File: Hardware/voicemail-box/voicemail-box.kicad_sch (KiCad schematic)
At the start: 13 parts, among them J1 Power, J2 Digital/PWM, J3 Analog, J4 Digital/PWM, J5 Conn_02x06_Top_Bottom, U1 ESP32-WROOM-32

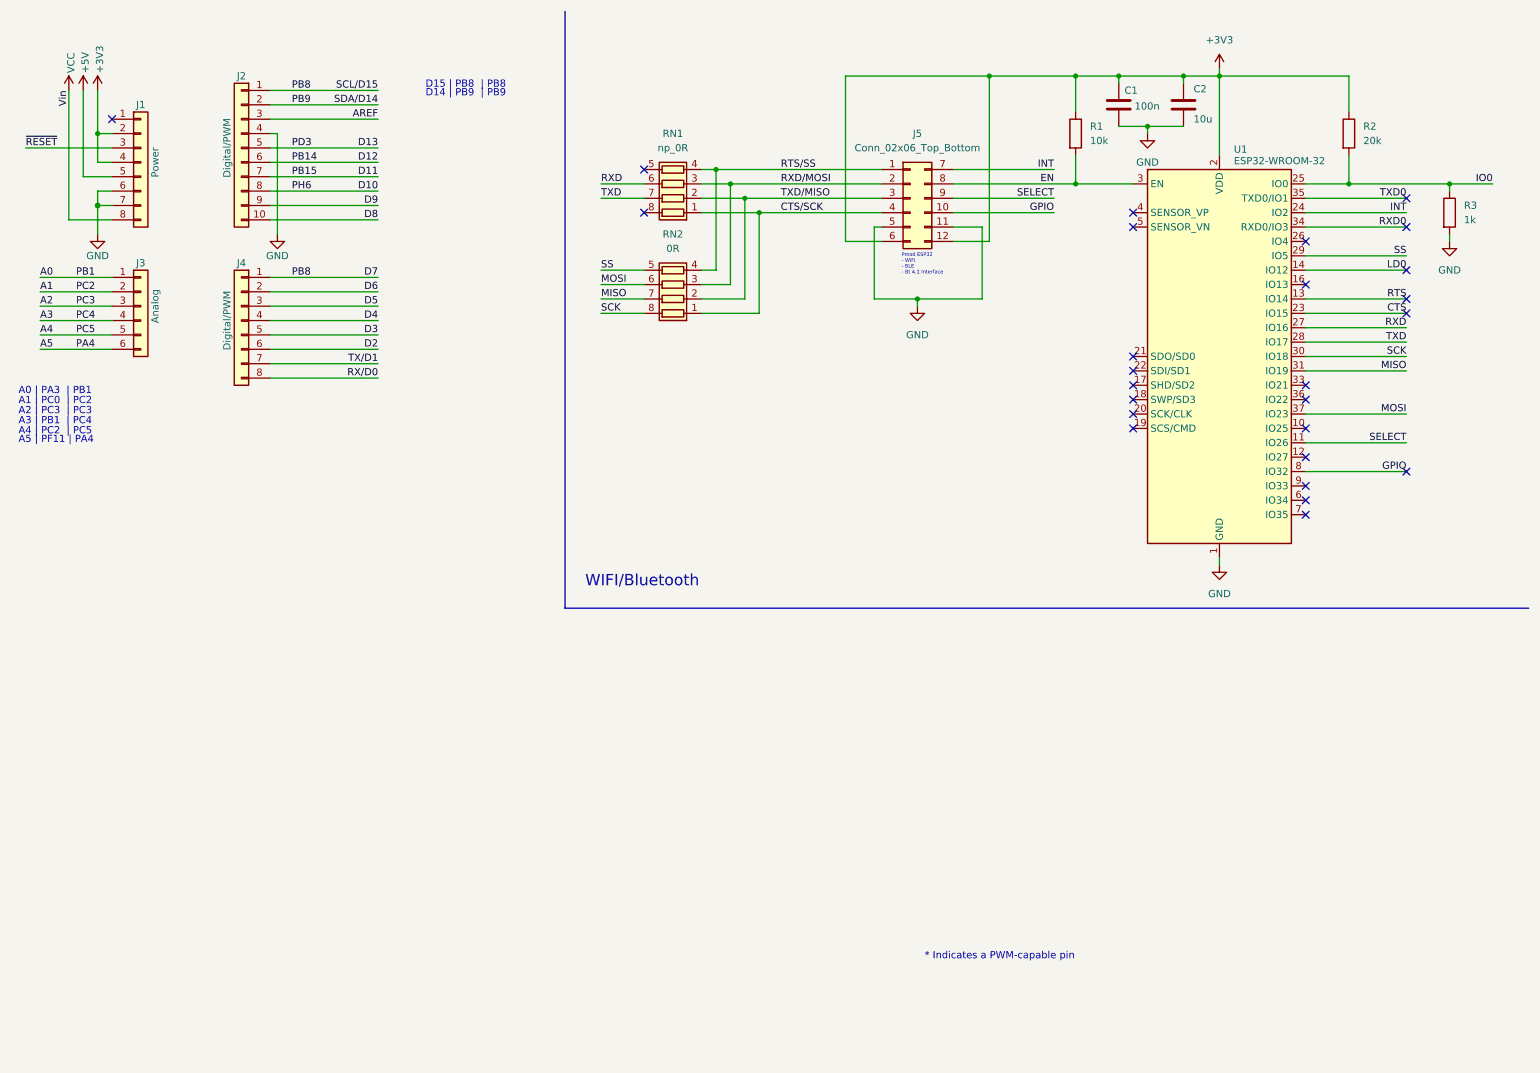
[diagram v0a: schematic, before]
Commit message: + gitignore ~ added existing pinout of sandbox tests
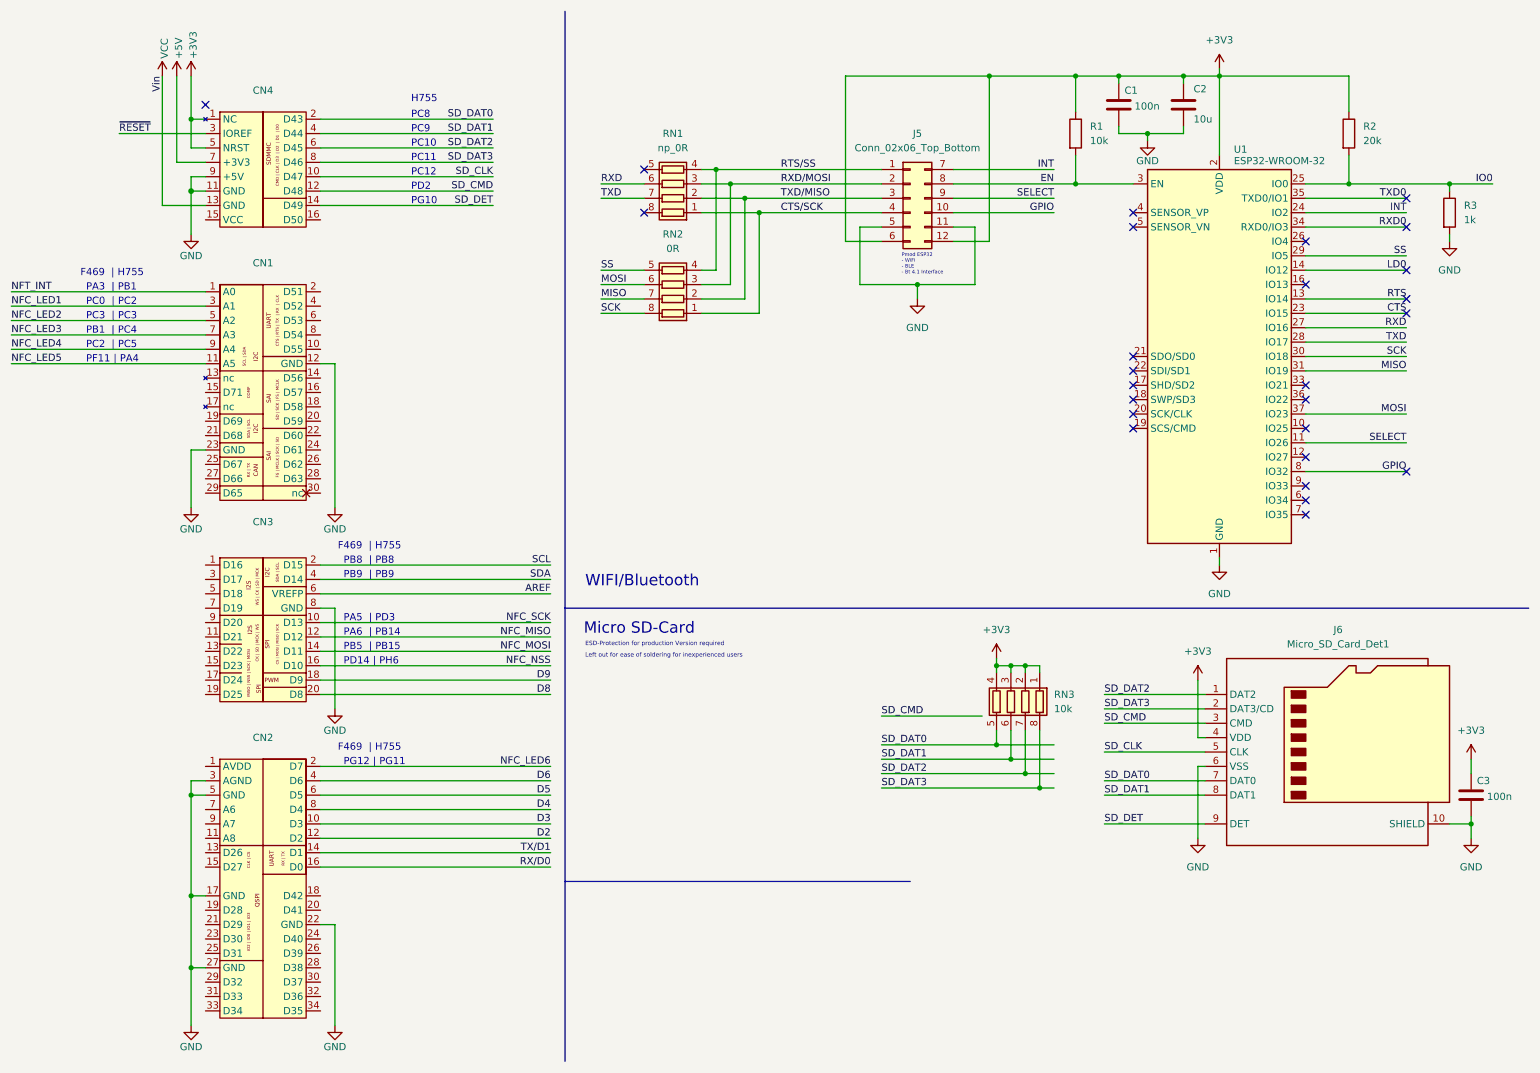
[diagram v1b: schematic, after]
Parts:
- removed J1: Power, Connector_PinSocket_2.54mm:PinSocket_1x08_P2.54mm_Vertical, symbol Connector_Generic:Conn_01x08
- removed J2: Digital/PWM, Connector_PinSocket_2.54mm:PinSocket_1x10_P2.54mm_Vertical, symbol Connector_Generic:Conn_01x10
- removed J3: Analog, Connector_PinSocket_2.54mm:PinSocket_1x06_P2.54mm_Vertical, symbol Connector_Generic:Conn_01x06
- removed J4: Digital/PWM, Connector_PinSocket_2.54mm:PinSocket_1x08_P2.54mm_Vertical, symbol Connector_Generic:Conn_01x08
- added C3: 100n, Capacitor_SMD:C_0805_2012Metric_Pad1.18x1.45mm_HandSolder, symbol Device:C
- added CN1: ~, Connector_PinSocket_2.54mm:PinSocket_2x15_P2.54mm_Vertical, symbol myParts:NUCLEO_144_Analog+
- added CN2: ~, Connector_PinSocket_2.54mm:PinSocket_2x17_P2.54mm_Vertical, symbol myParts:NUCLEO_144_GPIO+
- added CN3: ~, Connector_PinSocket_2.54mm:PinSocket_2x10_P2.54mm_Vertical, symbol myParts:NUCLEO_144_Periphery+
- added CN4: ~, Connector_PinSocket_2.54mm:PinSocket_2x08_P2.54mm_Vertical, symbol myParts:NUCLEO_144_Power
- added J6: Micro_SD_Card_Det1, symbol Connector:Micro_SD_Card_Det1
- added RN3: 10k, Resistor_SMD:R_Array_Convex_4x0603, symbol Device:R_Pack04
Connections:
- net +3V3: now also C3.1, CN4.1 (NC), CN4.5 (NRST), J6.4 (VDD), RN3.1 (R1.1), RN3.2 (R2.1), RN3.3 (R3.1), RN3.4 (R4.1)
- net +5V: now also CN4.7 (+3V3)
- net AREF: now also CN3.6 (VREFP)
- net D2: now also CN2.12 (D2)
- net D3: now also CN2.10 (D3)
- net D4: now also CN2.8 (D4)
- net D5: now also CN2.6 (D5)
- net D6: now also CN2.4 (D6)
- net D8: now also CN3.20 (D8)
- net D9: now also CN3.18 (D9)
- net GND: now also C3.2, CN1.12 (GND), CN1.23 (GND), CN2.17 (GND), CN2.22 (GND), CN2.27 (GND), CN2.3 (AGND), CN2.5 (GND), CN3.8 (GND), CN4.11 (GND), CN4.9 (+5V), J6.10 (SHIELD), J6.6 (VSS)
- net RX/D0: now also CN2.16 (D0)
- net TX/D1: now also CN2.14 (D1)
- net VCC: now also CN4.13 (GND)
- net ~{RESET}: now also CN4.3 (IOREF)
- new net NFC_LED1: CN1.3 (A1)
- new net NFC_LED2: CN1.5 (A2)
- new net NFC_LED3: CN1.7 (A3)
- new net NFC_LED4: CN1.9 (A4)
- new net NFC_LED5: CN1.11 (A5)
- new net NFC_LED6: CN2.2 (D7)
- new net NFC_MISO: CN3.12 (D12)
- new net NFC_MOSI: CN3.14 (D11)
- new net NFC_NSS: CN3.16 (D10)
- new net NFC_SCK: CN3.10 (D13)
- new net NFT_INT: CN1.1 (A0)
- new net SCL: CN3.2 (D15)
- new net SDA: CN3.4 (D14)
- new net SD_CLK: CN4.10 (D47), J6.5 (CLK)
- new net SD_CMD: CN4.12 (D48), J6.3 (CMD)
- new net SD_DAT0: CN4.2 (D43), J6.7 (DAT0), RN3.5 (R4.2)
- new net SD_DAT1: CN4.4 (D44), J6.8 (DAT1), RN3.6 (R3.2)
- new net SD_DAT2: CN4.6 (D45), J6.1 (DAT2), RN3.7 (R2.2)
- new net SD_DAT3: CN4.8 (D46), J6.2 (DAT3/CD), RN3.8 (R1.2)
- new net SD_DET: CN4.14 (D49), J6.9 (DET)
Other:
- note added: "ESD-Protection for production Version required"
- note added: "F469 | H755"
- note added: "H755"
- note added: "Left out for ease of soldering for inexperienced users"
- note added: "Micro SD-Card"
- note added: "PA3 | PB1"
- note added: "PA5 | PD3"
- note added: "PA6 | PB14"
- note added: "PB1 | PC4"
- note added: "PB5 | PB15"
- note added: "PB8 | PB8"
- note added: "PB9 | PB9"
- note added: "PC0 | PC2"
- note added: "PC10"
- note added: "PC11"
- note added: "PC12"
- note added: "PC2 | PC5"
- note added: "PC3 | PC3"
- note added: "PC8"
- note added: "PC9"
- note added: "PD14 | PH6"
- note added: "PD2"
- note added: "PF11 | PA4"
- note added: "PG10"
- note added: "PG12 | PG11"
- note removed: "* Indicates a PWM-capable pin"
- note removed: "A0 | PA3 | PB1"
- note removed: "A1 | PC0 | PC2"
- note removed: "A2 | PC3 | PC3"
- note removed: "A3 | PB1 | PC4"
- note removed: "A4 | PC2 | PC5"
- note removed: "A5 | PF11 | PA4"
- note removed: "D14 | PB9 | PB9"
- note removed: "D15 | PB8 | PB8"
